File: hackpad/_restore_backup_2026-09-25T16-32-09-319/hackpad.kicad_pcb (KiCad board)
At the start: 2 copper layers, 95.3 x 88.4 mm, 21 parts, among them SW1 SW_Push_45deg, SW10 RotaryEncoder_Switch, SW2 SW_Push_45deg, SW3 SW_Push_45deg, SW4 SW_Push_45deg, SW5 SW_Push_45deg, SW6 SW_Push_45deg, SW7 SW_Push_45deg, SW8 SW_Push_45deg, SW9 SW_Push_45deg, U1 MOUDLE-SEEEDUINO-XIAO, U2 ER_OLEDM0.91_1x-I2C

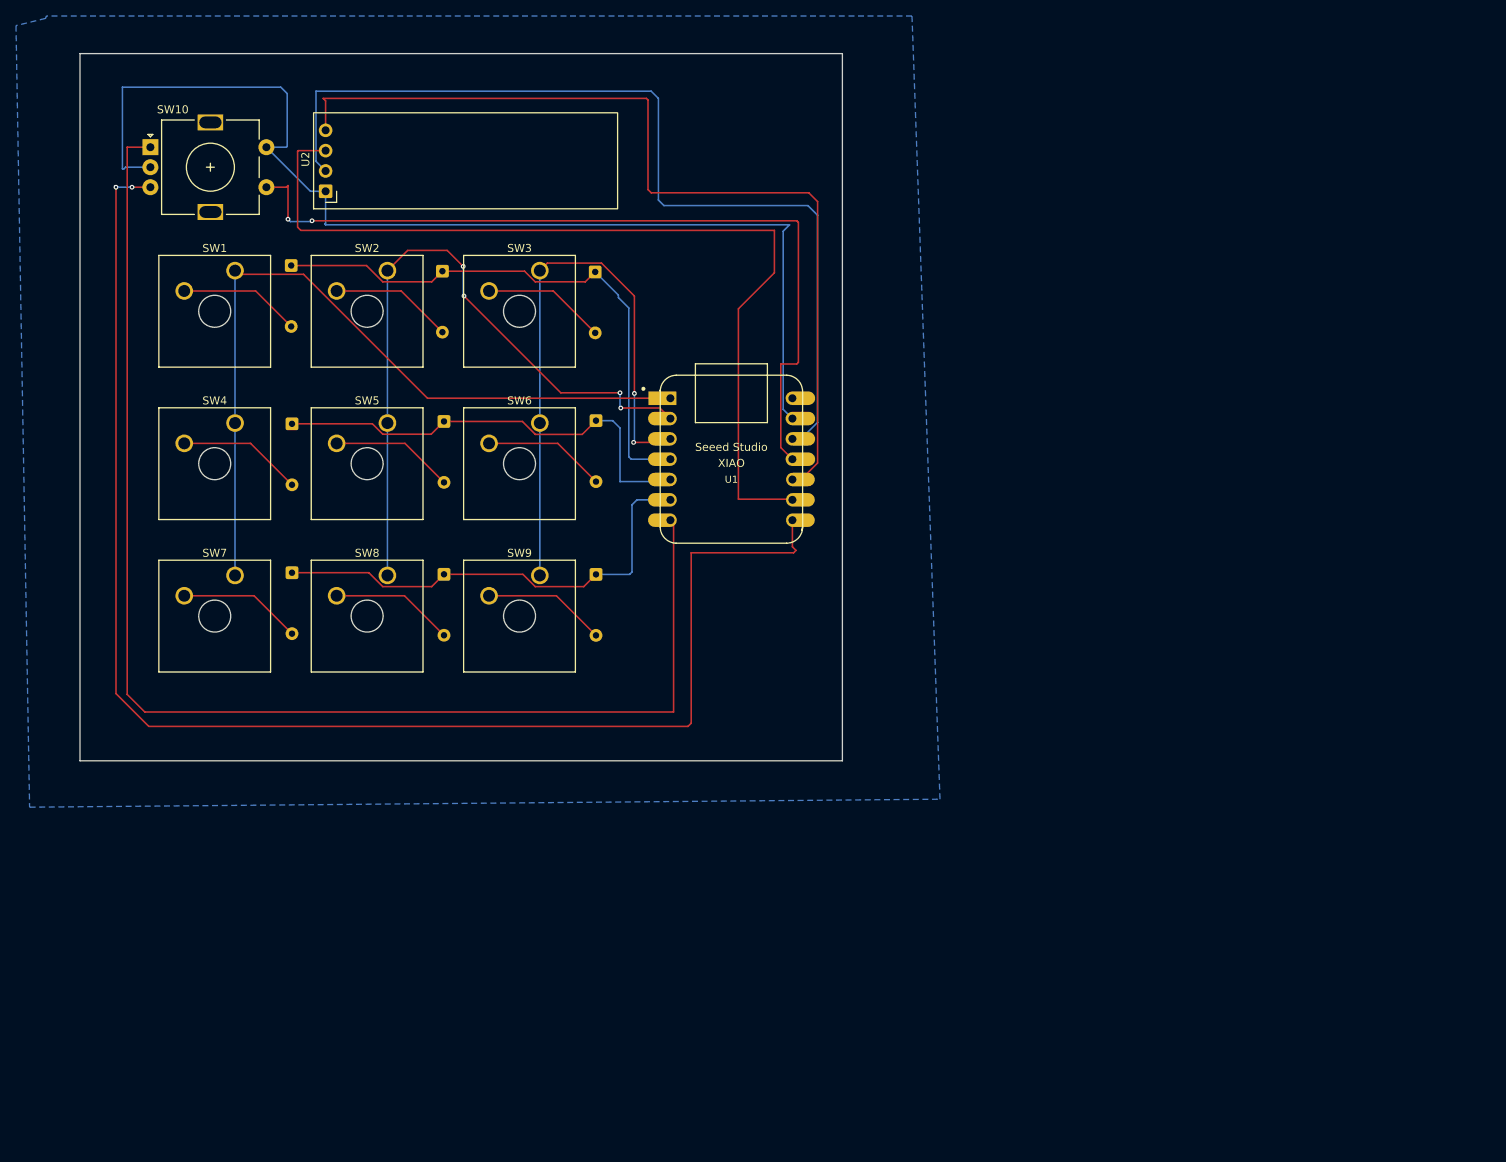
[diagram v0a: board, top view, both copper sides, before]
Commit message: Completed Routing and generated gerber files
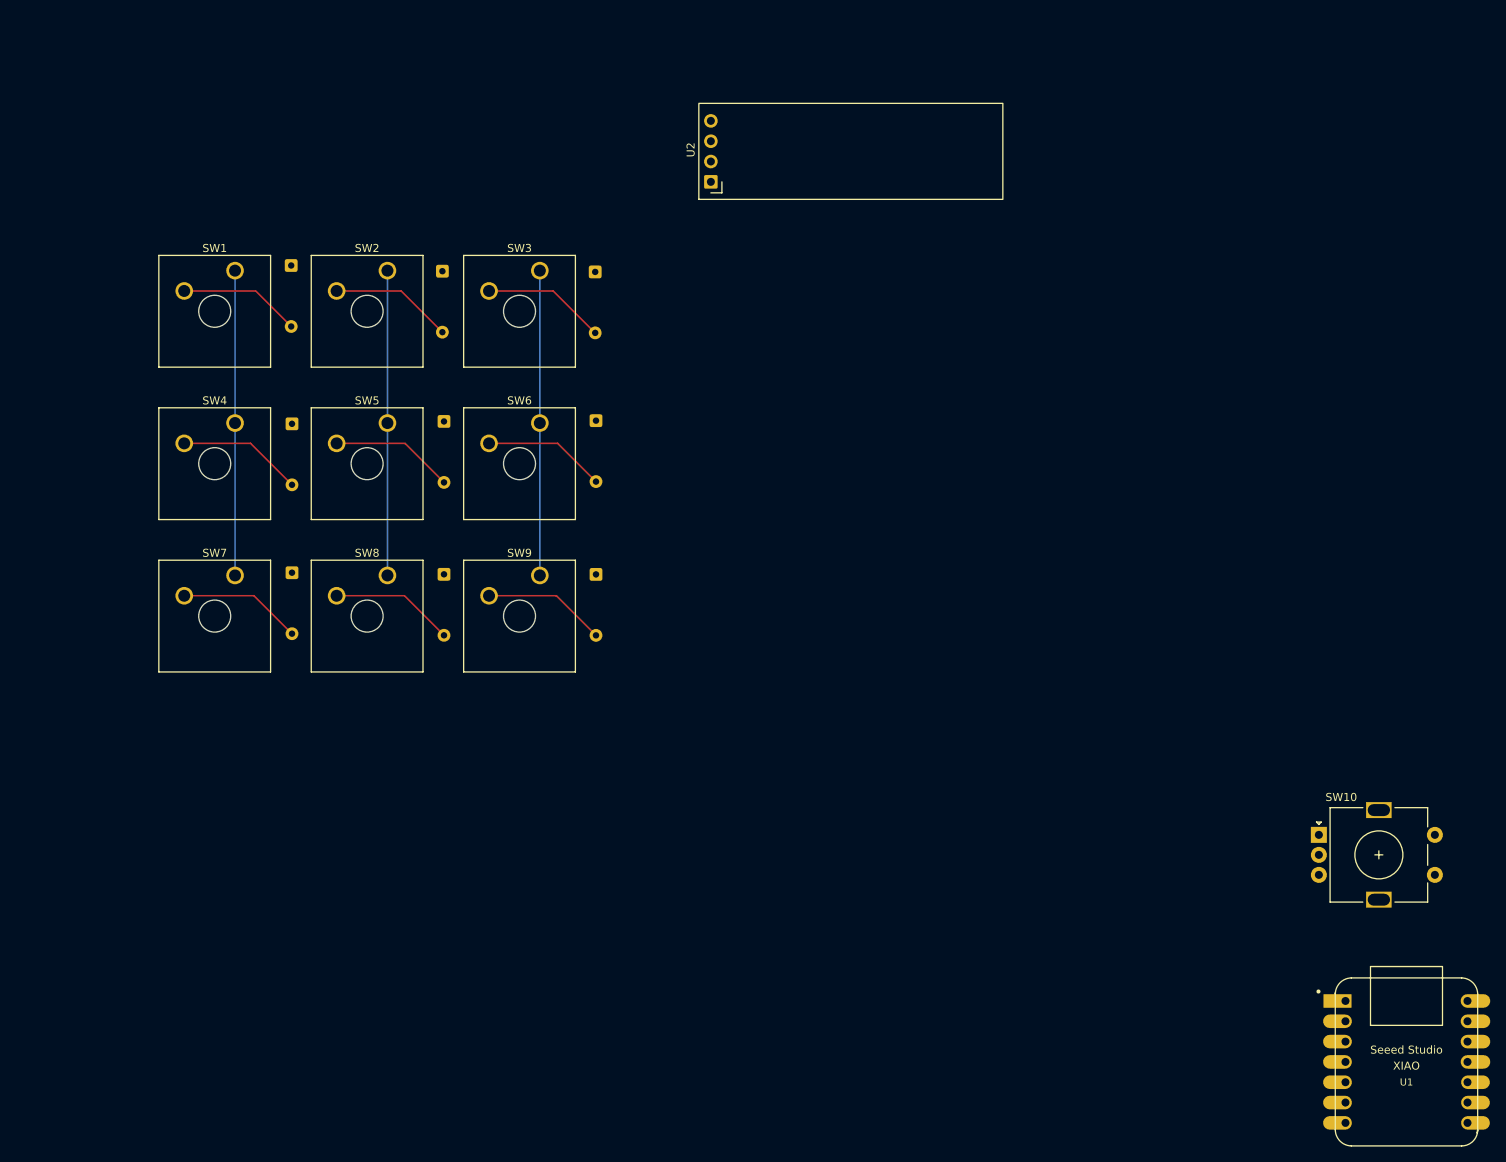
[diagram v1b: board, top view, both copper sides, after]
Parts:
- moved SW10 169.5 mm to (185.5, 120.5)
- moved U1 113.1 mm to (196.4, 148.9)
- moved U2 48.2 mm to (109.5, 38.9)
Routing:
- net Net-(U1-PB09_A7_D7_RX): track 180.9 -> 0.00 mm, vias 2 -> 0
- net Net-(U1-PB08_A6_D6_TX): track 164.7 -> 0.00 mm
- net GND: track 140.9 -> 0.00 mm
- net Net-(U1-3V3): track 116.9 -> 0.00 mm
- net Net-(U1-PA7_A8_D8_SCK): track 115.0 -> 0.00 mm
- net Net-(U1-PA5_A9_D9_MISO): track 114.5 -> 0.00 mm
- net Net-(U1-PA6_A10_D10_MOSI): track 103.3 -> 0.00 mm, vias 2 -> 0
- net Row 0: track 70.6 -> 0.00 mm
- net Column 0: track 99.1 -> 38.1 mm
- net Row 2: track 58.7 -> 0.00 mm
- net Row 1: track 57.1 -> 0.00 mm
- net Column 1: track 86.4 -> 38.1 mm, vias 4 -> 0
- net Column 2: track 75.1 -> 38.1 mm, vias 2 -> 0
- removed copper zone on B.Cu, net GND
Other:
- board outline removed
